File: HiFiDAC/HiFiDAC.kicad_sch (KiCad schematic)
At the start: 1 part, among them U2 PCM1794A

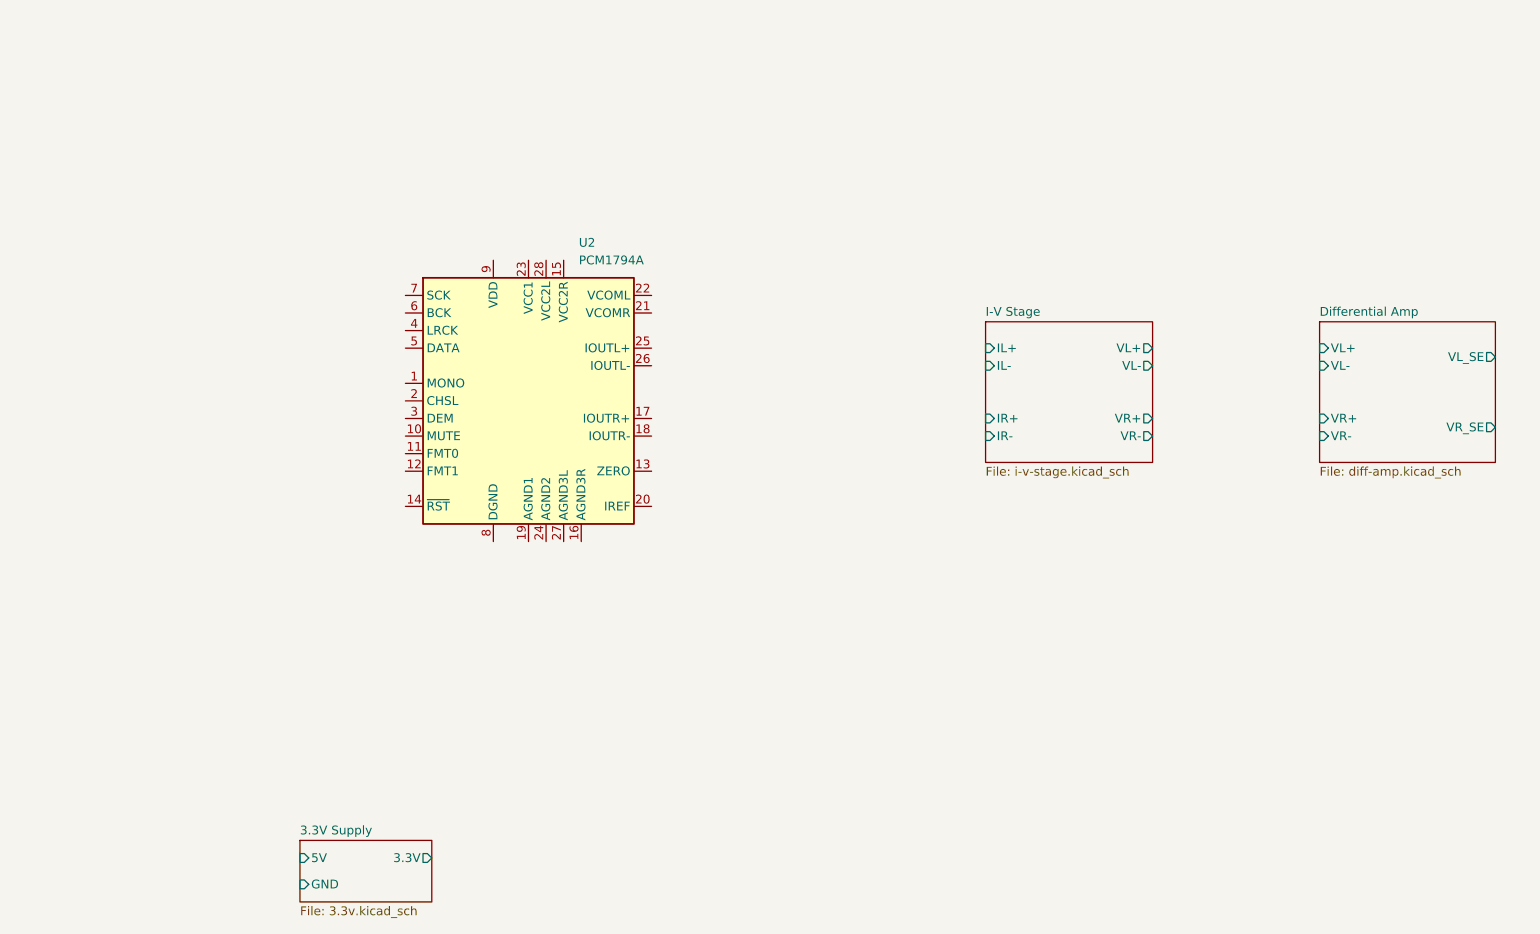
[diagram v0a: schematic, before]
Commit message: HiFiDAC progress
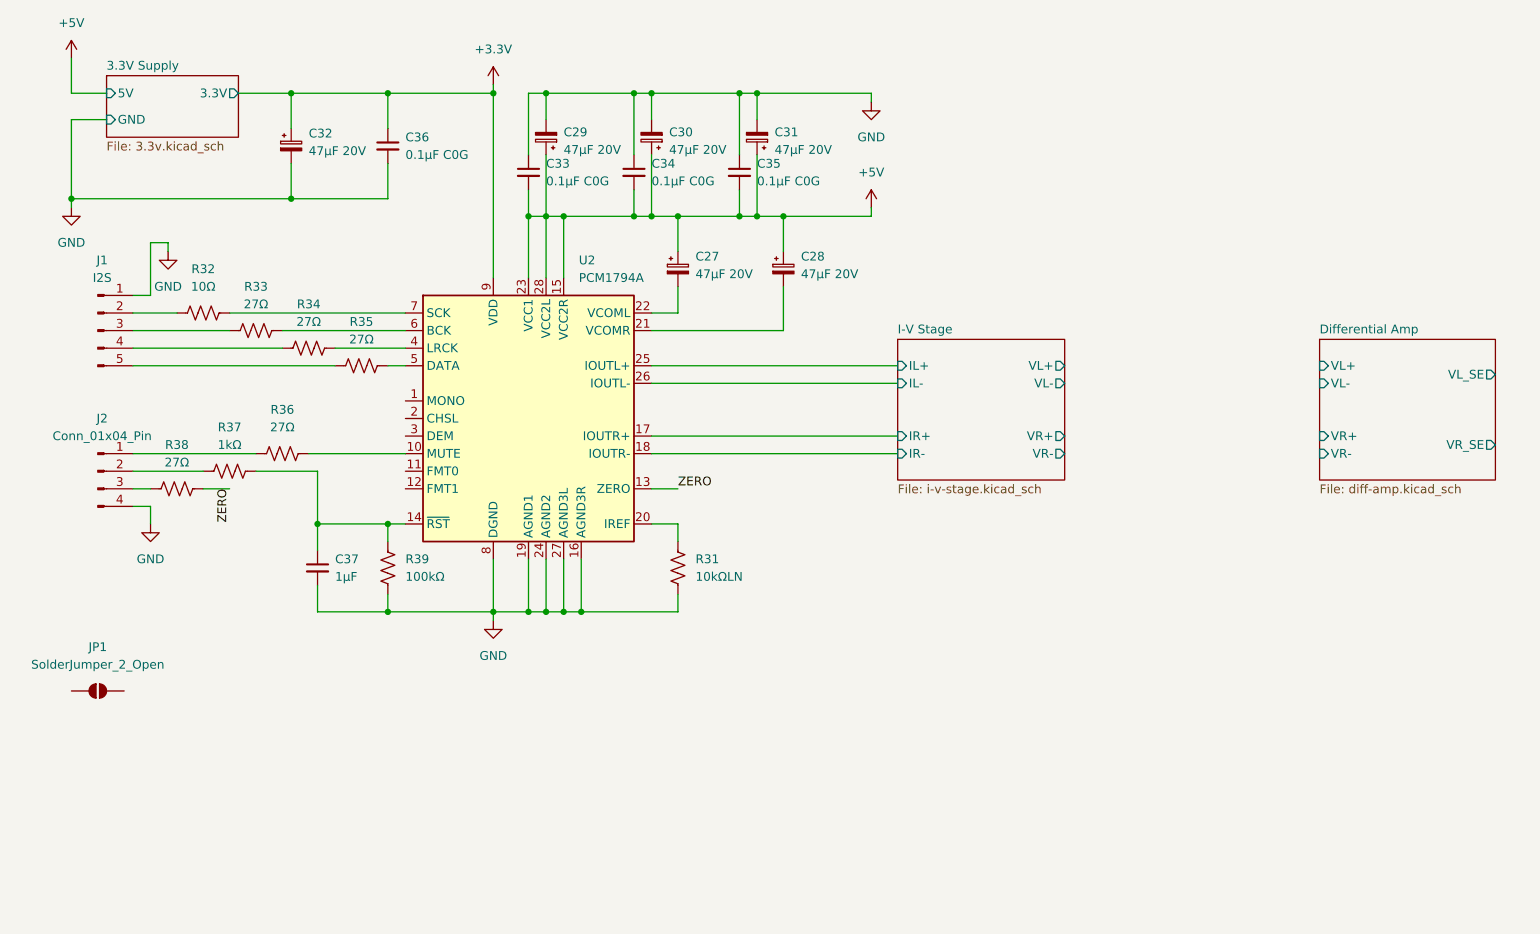
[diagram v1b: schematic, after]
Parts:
- added C27, C28, C29, C30, C31, C32: 47µF 20V, symbol Device:C_Polarized_Small
- added C33, C34, C35, C36: 0.1µF C0G, symbol Device:C_Small
- added C37: 1µF, symbol Device:C_Small
- added J1: I2S, symbol Connector:Conn_01x05_Pin
- added J2: Conn_01x04_Pin, symbol Connector:Conn_01x04_Pin
- added JP1: SolderJumper_2_Open, Jumper:SolderJumper-2_P1.3mm_Open_RoundedPad1.0x1.5mm, symbol Jumper:SolderJumper_2_Open
- added R31: 10kΩLN, symbol Device:R_US
- added R32: 10Ω, symbol Device:R_US
- added R33, R34, R35, R36, R38: 27Ω, symbol Device:R_US
- added R37: 1kΩ, symbol Device:R_US
- added R39: 100kΩ, symbol Device:R_US
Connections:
- net I-V Stage/IL+: now also U2.25 (IOUTL+)
- net I-V Stage/IL-: now also U2.26 (IOUTL-)
- net I-V Stage/IR+: now also U2.17 (IOUTR+)
- net I-V Stage/IR-: now also U2.18 (IOUTR-)
- net at U2.10 (MUTE): now also R36.2
- net ZERO: now reaches U2.13 (ZERO)
- net ZERO: now also R38.2
- net at U2.14 (~{RST}): now also C37.1, R37.2, R39.1
- net +5V: now reaches U2.15 (VCC2R)
- net +5V: now also U2.23 (VCC1), U2.28 (VCC2L), C27.1, C28.1, C29.1, C30.1, C31.1, C33.2, C34.2, C35.2
- net GND: now reaches U2.16 (AGND3R)
- net GND: now also U2.19 (AGND1), U2.24 (AGND2), U2.27 (AGND3L), U2.8 (DGND), C29.2, C30.2, C31.2, C32.2, C33.1, C34.1, C35.1, C36.2, C37.2, J1.1 (Pin_1), J2.4 (Pin_4), R31.2, R39.2
- net at U2.20 (IREF): now also R31.1
- net at U2.21 (VCOMR): now also C28.2
- net at U2.22 (VCOML): now also C27.2
- net at U2.4 (LRCK): now also R34.2
- net at U2.5 (DATA): now also R35.2
- net at U2.6 (BCK): now also R33.2
- net at U2.7 (SCK): now also R32.2
- net +3.3V: now reaches U2.9 (VDD)
- net +3.3V: now also C32.1, C36.1
- new net: J2.3 (Pin_3), R38.1
- new net: J1.4 (Pin_4), R34.1
- new net: J2.1 (Pin_1), R36.1
- new net: J2.2 (Pin_2), R37.1
- new net: J1.2 (Pin_2), R32.1
- new net: J1.3 (Pin_3), R33.1
- new net: J1.5 (Pin_5), R35.1
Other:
- moved on the sheet: U2
